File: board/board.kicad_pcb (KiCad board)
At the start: 4 copper layers, 29 x 13 mm, 8 parts, among them J1 osf.011, J2 osf.011

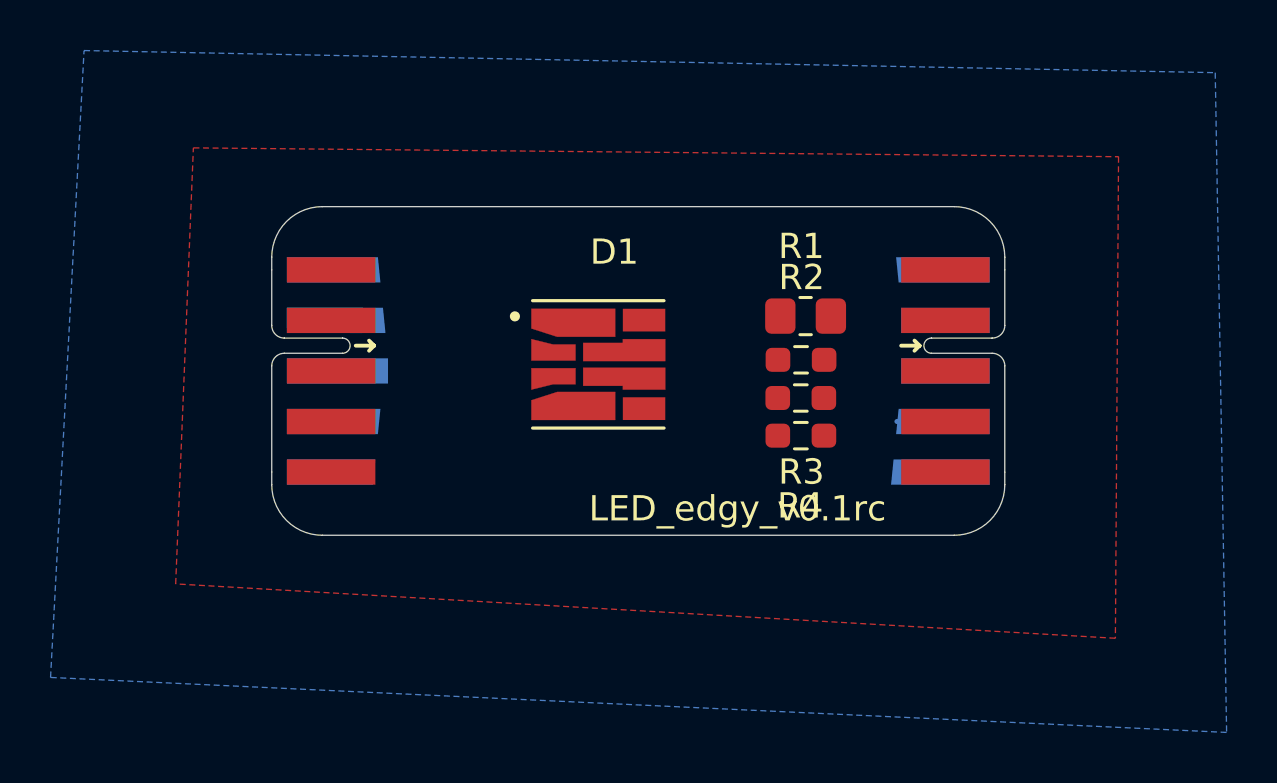
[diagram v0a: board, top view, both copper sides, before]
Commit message: Save changes
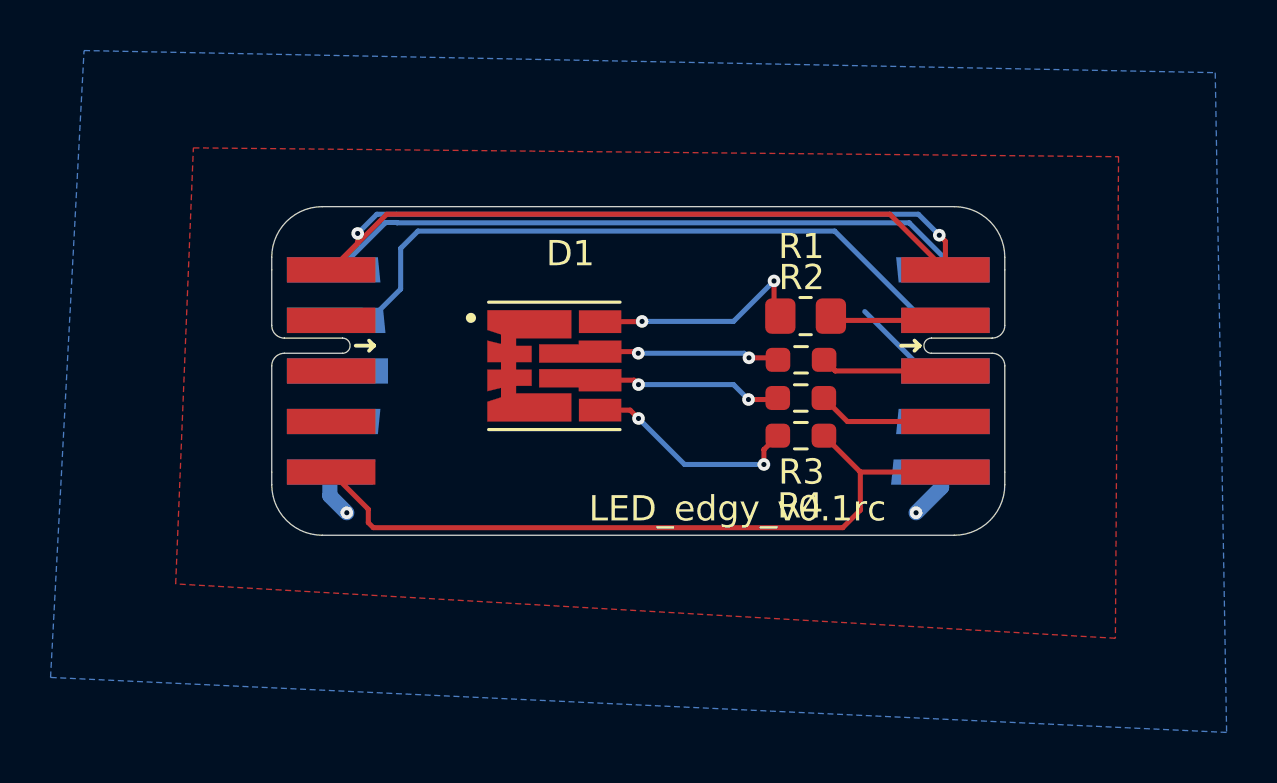
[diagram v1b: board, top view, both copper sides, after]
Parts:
- moved D1 1.74 mm to (151.2, 96.3)
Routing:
- net Net-(J1-GND-Pad1): track 0.03 -> 53.1 mm, vias 0 -> 2
- net Net-(J1-GPIO3): track 0.38 -> 29.7 mm
- net Net-(J1-GPIO5): track 1.55 -> 30.0 mm
- net Net-(J1-GPIO4): track 0.00 -> 26.0 mm
- net Net-(D1-Pad8): track 0.00 -> 9.35 mm, vias 0 -> 2
- net Net-(D1-Pad5): track 0.00 -> 8.74 mm, vias 0 -> 2
- net Net-(D1-Pad7): track 0.00 -> 7.63 mm, vias 0 -> 2
- net Net-(J1-5V): track 0.00 -> 7.42 mm, vias 0 -> 2
- net Net-(D1-Pad6): track 0.00 -> 7.37 mm, vias 0 -> 2
- net Net-(J1-GPIO2): track 0.00 -> 5.19 mm
- net Net-(J1-GPIO1): track 0.00 -> 4.98 mm
- net Net-(J1-GPIO0): track 0.00 -> 4.60 mm
- net Net-(J1-GND-Pad8): track 0.83 -> 4.99 mm
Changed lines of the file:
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@@
   )
   (footprint "GW_J9LHS1:LED_GW_J9LHS1.4M-C1C7-2+58+MQ+30A-1-100-R33" (layer "F.Cu")
-    (at 152.92 96.24)
+    (at 151.18 96.3)
     (property "MANUFACTURER" "OSRAM Opto Semiconductors")
     (property "MAXIMUM_PACKAGE_HEIGHT" "1.2 mm")
@@
     (effects (font (size 1 1) (thickness 0.15)))
   )
-  (segment (start 166.65 92.475) (end 166.65 92.5) (width 0.2) (layer "F.Cu") (net 6))
+  (segment (start 149.37 95.8) (end 149.37 96.8) (width 0.6) (layer "F.Cu") (net 1))
+  (segment (start 149.37 96.8) (end 149.37 98.05) (width 0.6) (layer "F.Cu") (net 1))
+  (segment (start 149.37 95.8) (end 149.37 94.55) (width 0.6) (layer "F.Cu") (net 1))
+  (via (at 142.97 102.11) (size 0.5) (drill 0.2) (layers "F.Cu" "B.Cu") (net 1))
+  (via (at 165.49 102.11) (size 0.5) (drill 0.2) (layers "F.Cu" "B.Cu") (net 1))
+  (segment (start 142.3 101.44) (end 142.97 102.11) (width 0.6) (layer "B.Cu") (net 1))
+  (segment (start 166.5 101.1) (end 165.49 102.11) (width 0.6) (layer "B.Cu") (net 1))
+  (segment (start 142.3 100.5) (end 142.3 101.44) (width 0.6) (layer "B.Cu") (net 1))
+  (segment (start 166.5 100.5) (end 166.5 101.1) (width 0.6) (layer "B.Cu") (net 1))
+  (segment (start 159.9475 95.98) (end 160.0275 96.06) (width 0.2) (layer "F.Cu") (net 2))
+  (segment (start 152.99 95.735) (end 154.435 95.735) (width 0.2) (layer "F.Cu") (net 2))
+  (segment (start 158.88 95.98) (end 159.9475 95.98) (width 0.2) (layer "F.Cu") (net 2))
+  (segment (start 159.7025 95.735) (end 160.0275 96.06) (width 0.2) (layer "F.Cu") (net 2))
+  (segment (start 154.435 95.735) (end 154.5 95.8) (width 0.2) (layer "F.Cu") (net 2))
+  (via (at 154.5 95.8) (size 0.5) (drill 0.2) (layers "F.Cu" "B.Cu") (net 2))
+  (via (at 158.88 95.98) (size 0.5) (drill 0.2) (layers "F.Cu" "B.Cu") (net 2))
+  (segment (start 158.7 95.8) (end 158.88 95.98) (width 0.2) (layer "B.Cu") (net 2))
+  (segment (start 154.5 95.8) (end 158.7 95.8) (width 0.2) (layer "B.Cu") (net 2))
+  (segment (start 159.47 99.61) (end 160.02 99.06) (width 0.2) (layer "F.Cu") (net 3))
+  (segment (start 154.18 98.05) (end 154.51 98.38) (width 0.2) (layer "F.Cu") (net 3))
+  (segment (start 152.99 98.05) (end 154.18 98.05) (width 0.2) (layer "F.Cu") (net 3))
+  (segment (start 159.47 100.2) (end 159.47 99.61) (width 0.2) (layer "F.Cu") (net 3))
+  (via (at 159.47 100.2) (size 0.5) (drill 0.2) (layers "F.Cu" "B.Cu") (net 3))
+  (via (at 154.51 98.38) (size 0.5) (drill 0.2) (layers "F.Cu" "B.Cu") (net 3))
+  (segment (start 156.33 100.2) (end 159.47 100.2) (width 0.2) (layer "B.Cu") (net 3))
+  (segment (start 154.51 98.38) (end 156.33 100.2) (width 0.2) (layer "B.Cu") (net 3))
+  (segment (start 159.9575 97.63) (end 160.0175 97.57) (width 0.2) (layer "F.Cu") (net 4))
+  (segment (start 152.99 96.865) (end 154.335 96.865) (width 0.2) (layer "F.Cu") (net 4))
+  (segment (start 154.335 96.865) (end 154.51 97.04) (width 0.2) (layer "F.Cu") (net 4))
+  (segment (start 158.86 97.63) (end 159.9575 97.63) (width 0.2) (layer "F.Cu") (net 4))
+  (via (at 158.86 97.63) (size 0.5) (drill 0.2) (layers "F.Cu" "B.Cu") (net 4))
+  (via (at 154.51 97.04) (size 0.5) (drill 0.2) (layers "F.Cu" "B.Cu") (net 4))
+  (segment (start 158.27 97.04) (end 158.86 97.63) (width 0.2) (layer "B.Cu") (net 4))
+  (segment (start 154.51 97.04) (end 158.27 97.04) (width 0.2) (layer "B.Cu") (net 4))
+  (segment (start 152.99 94.55) (end 154.64 94.55) (width 0.2) (layer "F.Cu") (net 5))
+  (segment (start 154.64 94.55) (end 154.65 94.54) (width 0.2) (layer "F.Cu") (net 5))
+  (segment (start 159.87 94.08) (end 160.12 94.33) (width 0.2) (layer "F.Cu") (net 5))
+  (segment (start 159.9 94.55) (end 160.12 94.33) (width 0.2) (layer "F.Cu") (net 5))
+  (segment (start 159.87 92.94) (end 159.87 94.08) (width 0.2) (layer "F.Cu") (net 5))
+  (via (at 159.87 92.94) (size 0.5) (drill 0.2) (layers "F.Cu" "B.Cu") (net 5))
+  (via (at 154.65 94.54) (size 0.5) (drill 0.2) (layers "F.Cu" "B.Cu") (net 5))
+  (segment (start 158.27 94.54) (end 159.87 92.94) (width 0.2) (layer "B.Cu") (net 5))
+  (segment (start 154.65 94.54) (end 158.27 94.54) (width 0.2) (layer "B.Cu") (net 5))
+  (segment (start 143.4 91.06) (end 143.4 91.45) (width 0.2) (layer "F.Cu") (net 6))
+  (segment (start 166.65 92.5) (end 166.65 91.37) (width 0.2) (layer "F.Cu") (net 6))
+  (segment (start 142.35 92.5) (end 144.55 90.3) (width 0.2) (layer "F.Cu") (net 6))
+  (segment (start 164.45 90.3) (end 166.65 92.5) (width 0.2) (layer "F.Cu") (net 6))
+  (segment (start 144.55 90.3) (end 164.45 90.3) (width 0.2) (layer "F.Cu") (net 6))
+  (segment (start 166.65 91.37) (end 166.41 91.13) (width 0.2) (layer "F.Cu") (net 6))
+  (segment (start 143.4 91.45) (end 142.35 92.5) (width 0.2) (layer "F.Cu") (net 6))
+  (via (at 143.4 91.06) (size 0.5) (drill 0.2) (layers "F.Cu" "B.Cu") (net 6))
+  (via (at 166.41 91.13) (size 0.5) (drill 0.2) (layers "F.Cu" "B.Cu") (net 6))
+  (segment (start 144.16 90.3) (end 143.4 91.06) (width 0.2) (layer "B.Cu") (net 6))
+  (segment (start 144.94 90.3) (end 144.16 90.3) (width 0.2) (layer "B.Cu") (net 6))
+  (segment (start 165.58 90.3) (end 144.94 90.3) (width 0.2) (layer "B.Cu") (net 6))
+  (segment (start 166.41 91.13) (end 165.58 90.3) (width 0.2) (layer "B.Cu") (net 6))
+  (segment (start 162.12 94.33) (end 162.29 94.5) (width 0.2) (layer "F.Cu") (net 7))
+  (segment (start 162.29 94.5) (end 166.65 94.5) (width 0.2) (layer "F.Cu") (net 7))
+  (segment (start 162.2925 96.5) (end 166.65 96.5) (width 0.2) (layer "F.Cu") (net 8))
+  (segment (start 161.8525 96.06) (end 162.2925 96.5) (width 0.2) (layer "F.Cu") (net 8))
+  (segment (start 161.8425 97.57) (end 162.7725 98.5) (width 0.2) (layer "F.Cu") (net 9))
+  (segment (start 162.7725 98.5) (end 166.65 98.5) (width 0.2) (layer "F.Cu") (net 9))
   (segment (start 142.725 100.5) (end 142.35 100.5) (width 0.2) (layer "F.Cu") (net 10))
+  (segment (start 163.285 102.005) (end 163.285 100.5) (width 0.2) (layer "F.Cu") (net 10))
+  (segment (start 161.845 99.06) (end 163.285 100.5) (width 0.2) (layer "F.Cu") (net 10))
+  (segment (start 143.82 101.97) (end 143.82 102.5) (width 0.2) (layer "F.Cu") (net 10))
+  (segment (start 143.82 102.5) (end 144.02 102.7) (width 0.2) (layer "F.Cu") (net 10))
+  (segment (start 142.35 100.5) (end 143.82 101.97) (width 0.2) (layer "F.Cu") (net 10))
+  (segment (start 162.59 102.7) (end 163.285 102.005) (width 0.2) (layer "F.Cu") (net 10))
+  (segment (start 163.285 100.5) (end 166.65 100.5) (width 0.2) (layer "F.Cu") (net 10))
+  (segment (start 144.02 102.7) (end 162.59 102.7) (width 0.2) (layer "F.Cu") (net 10))
+  (segment (start 165.22 90.64) (end 144.96 90.64) (width 0.2) (layer "B.Cu") (net 11))
+  (segment (start 144.96 90.64) (end 144.947 90.627) (width 0.2) (layer "B.Cu") (net 11))
+  (segment (start 144.48 90.65458) (end 142.63458 92.5) (width 0.2) (layer "B.Cu") (net 11))
+  (segment (start 166.6 92.5) (end 166.6 92.02) (width 0.2) (layer "B.Cu") (net 11))
+  (segment (start 166.6 92.02) (end 165.22 90.64) (width 0.2) (layer "B.Cu") (net 11))
+  (segment (start 144.48 90.627) (end 144.48 90.65458) (width 0.2) (layer "B.Cu") (net 11))
+  (segment (start 142.63458 92.5) (end 142.4 92.5) (width 0.2) (layer "B.Cu") (net 11))
+  (segment (start 144.947 90.627) (end 144.48 90.627) (width 0.2) (layer "B.Cu") (net 11))
+  (segment (start 162.27 90.967) (end 165.803 94.5) (width 0.2) (layer "B.Cu") (net 12))
   (segment (start 166.65 94.5) (end 165.1 94.5) (width 0.2) (layer "B.Cu") (net 12))
+  (segment (start 145.783 90.967) (end 162.27 90.967) (width 0.2) (layer "B.Cu") (net 12))
+  (segment (start 145.1 93.26) (end 145.1 91.65) (width 0.2) (layer "B.Cu") (net 12))
+  (segment (start 143.86 94.5) (end 145.1 93.26) (width 0.2) (layer "B.Cu") (net 12))
+  (segment (start 142.1 94.5) (end 143.86 94.5) (width 0.2) (layer "B.Cu") (net 12))
+  (segment (start 165.803 94.5) (end 166.65 94.5) (width 0.2) (layer "B.Cu") (net 12))
+  (segment (start 145.1 91.65) (end 145.783 90.967) (width 0.2) (layer "B.Cu") (net 12))
   (segment (start 166.65 96.5) (end 165.825 96.5) (width 0.2) (layer "B.Cu") (net 13))
+  (segment (start 166.65 96.5) (end 165.81 96.5) (width 0.2) (layer "B.Cu") (net 13))
+  (segment (start 165.81 96.5) (end 163.46 94.15) (width 0.2) (layer "B.Cu") (net 13))
   (segment (start 166.6 98.5) (end 164.732948 98.5) (width 0.2) (layer "B.Cu") (net 14))
   (zone (net 1) (net_name "Net-(J1-5V)") (layer "F.Cu") (hatch edge 0.508)

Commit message: Update PCB Design | Add routes
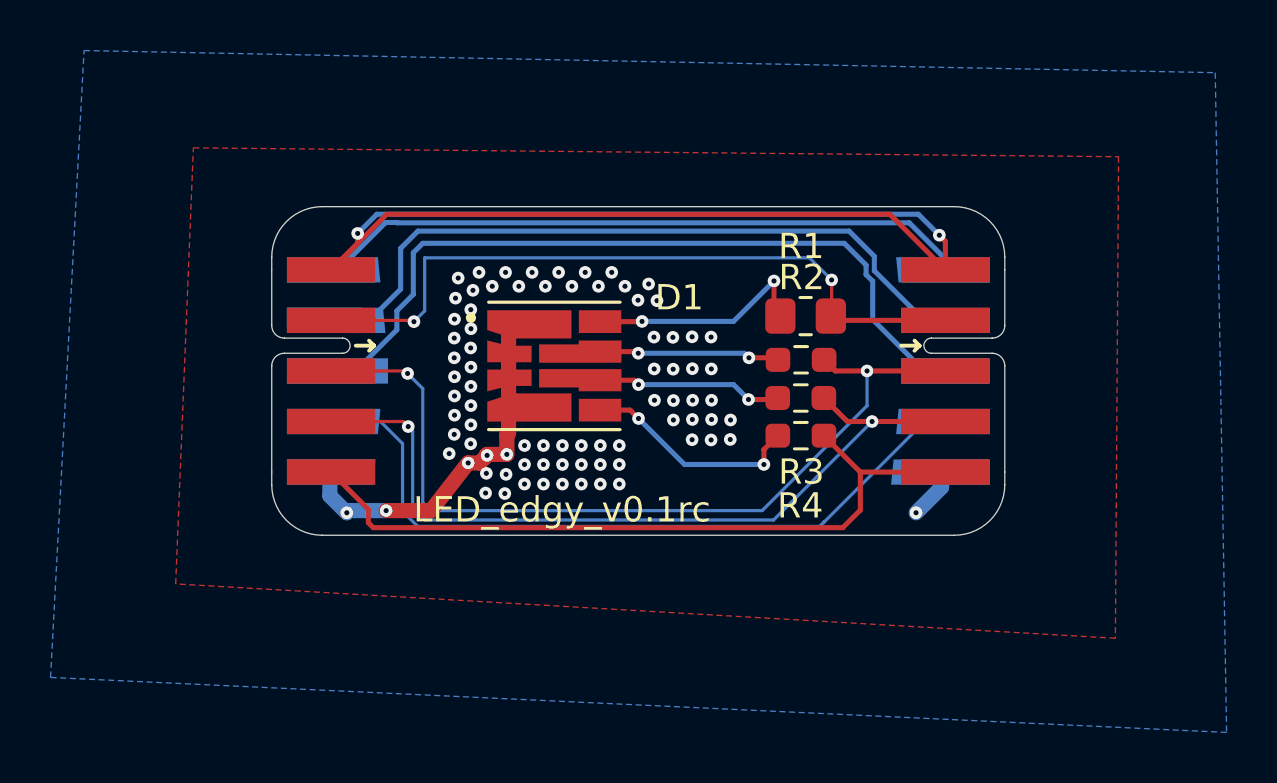
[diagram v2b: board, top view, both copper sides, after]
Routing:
- net Net-(J1-GPIO1): track 4.98 -> 34.2 mm, vias 0 -> 2
- net Net-(J1-3.3V): track 1.87 -> 29.2 mm
- net Net-(J1-GND-Pad8): track 4.99 -> 31.6 mm
- net Net-(J1-GPIO2): track 5.19 -> 31.6 mm, vias 0 -> 2
- net Net-(J1-GPIO0): track 4.60 -> 28.5 mm, vias 0 -> 2
- net Net-(J1-5V): track 7.42 -> 16.7 mm, vias 2 -> 81
- net Net-(J1-GPIO5): track 30.0 -> 28.8 mm
